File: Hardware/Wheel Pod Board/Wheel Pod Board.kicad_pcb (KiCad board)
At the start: 2 copper layers, 90 x 25.4 mm, 32 parts, among them J1 Conn_RJ-45, P1 Stepper, P2 RS232, P3 SWD, P4 SyRen, P5 BATT, U1 STM32F401RCT6, X1 24MHz

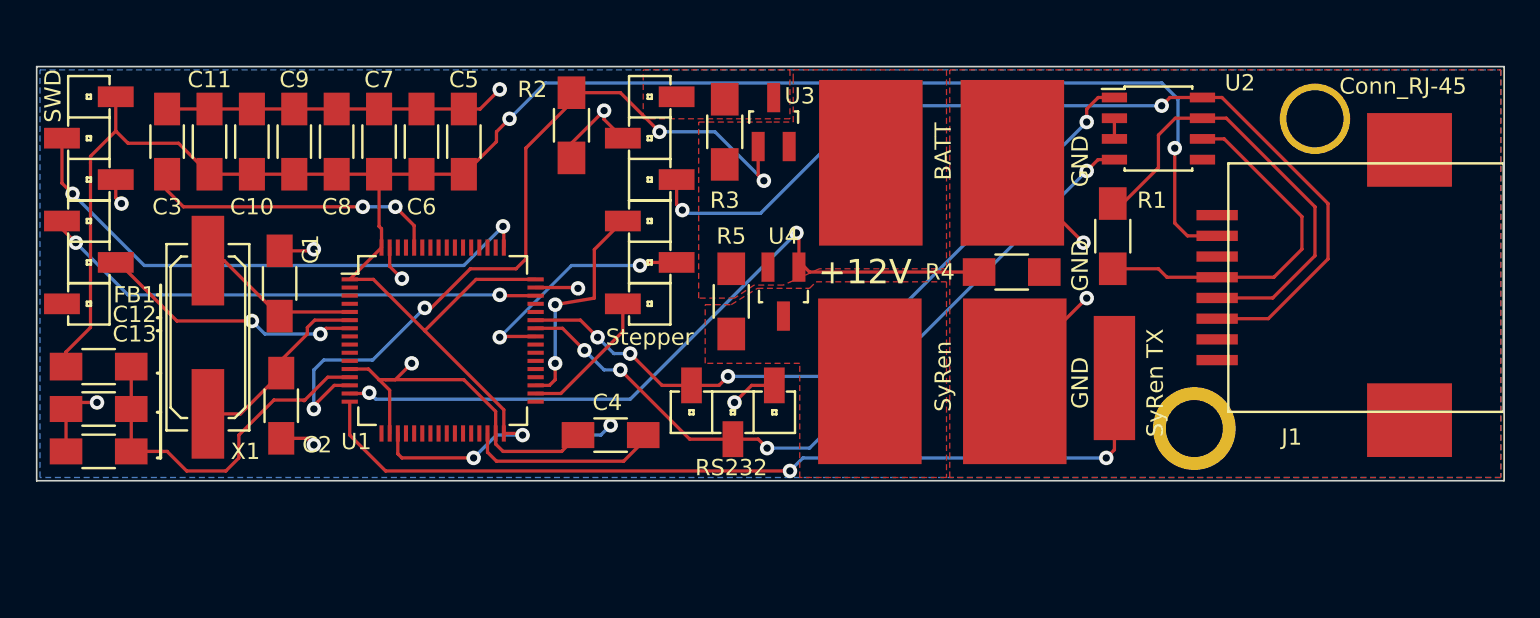
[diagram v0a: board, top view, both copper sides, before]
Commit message: Progress on new pcb route
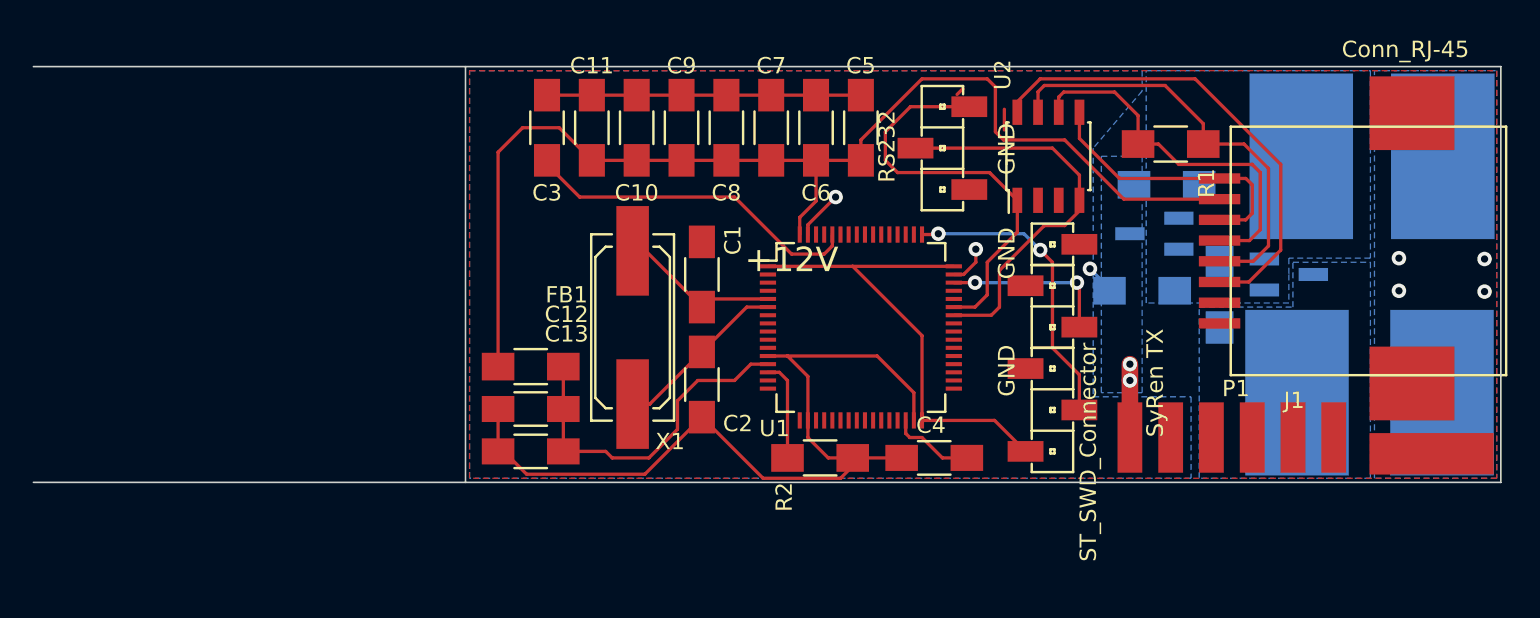
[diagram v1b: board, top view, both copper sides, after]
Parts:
- removed MountingHole_3-5mm (x2): VAL**, MAVRIC_footprints:PlatedMountingHole_3-5mm
- C4: value w4.7uF -> 4.7uF
- P1: value Stepper -> UIM240XX_Stepper_Conn; footprint MAVRIC_footprints:1x6_SMD_header -> MAVRIC_footprints:SolderWirePad_6xInline_0-8mmDrill
- P3: value SWD -> ST_SWD_Connector
- P4, P5, R3, R4, R5: moved to B.Cu
- U2: value (none) -> SN75176BDR
- U3, U4: value (none) -> ZXCT1107; moved to B.Cu
- moved P3 59.8 mm to (255.7, 146.1), turned to 90 degrees
- moved P1 38.3 mm to (266.4, 151.6), turned to 0 degrees
- moved U4 31.0 mm to (270.2, 141.6), turned to 90 degrees
- moved R5 30.0 mm to (265.9, 142.8)
- moved R3 27.3 mm to (262.7, 136.1), turned to 180 degrees
- moved C12 26.5 mm to (223.7, 149.8)
- moved C13 26.5 mm to (223.7, 152.4)
- moved FB1 26.5 mm to (223.7, 147.2)
- moved P5 26.4 mm to (277.7, 134.3)
- moved P4 26.2 mm to (270.7, 148.8)
- moved X1 26.1 mm to (229.9, 144.8)
- moved C1 25.9 mm to (234.2, 141.6)
- moved C2 25.8 mm to (234.2, 148.3)
- moved U1 25.7 mm to (243.9, 144.8)
- moved R2 25.5 mm to (241.4, 152.8), turned to 180 degrees
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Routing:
- net /USART2_TX: track 54.8 -> 0.00 mm, vias 2 -> 0
- net /SyRenCurrent: track 45.1 -> 0.00 mm, vias 2 -> 0
- net /StepperCurrent: track 48.8 -> 6.16 mm, vias 4 -> 0
- net +3V3: track 138.2 -> 101.0 mm, vias 4 -> 0
- net +5V: track 59.1 -> 29.4 mm, vias 2 -> 0
- net /USART1_TX: track 45.9 -> 24.6 mm, vias 4 -> 0
- net /SWDIO: track 31.2 -> 10.3 mm
- net /USART1_RX: track 44.9 -> 25.6 mm, vias 4 -> 0
- net /NRST: track 16.3 -> 0.00 mm, vias 2 -> 0
- net /SWCLK: track 34.2 -> 18.5 mm
- net /Step_Step: track 15.0 -> 0.00 mm, vias 2 -> 0
- net /Step_Direction: track 13.8 -> 0.00 mm, vias 2 -> 0
- net GND: track 86.5 -> 96.7 mm, vias 12 -> 7
- net /Step_Enable: track 8.62 -> 0.00 mm
- net Net-(C4-Pad1): track 11.8 -> 5.17 mm
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- added copper zone on B.Cu, net +12V
- added copper zone on B.Cu, net /Stp+12V
- added copper zone on B.Cu, net Net-(P4-Pad2)
- removed copper zone on F.Cu, net +12V
- removed copper zone on F.Cu, net /Stp+12V
- removed copper zone on F.Cu, net Net-(P4-Pad2)
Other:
- board size 90 x 25.4 mm -> 90 x 25.5 mm
